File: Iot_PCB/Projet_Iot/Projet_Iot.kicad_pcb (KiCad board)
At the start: 2 copper layers, 27 parts, among them J11 110990030, J14 110990030, J17 110990030, J18 110990030, J23 110990030, J24 110990030, J36 110990030, J38 110990030, J40 110990030, J42 110990030, J8 110990030, J9 110990030, U11 FDC6326L, U6 uPesy_ESP32_Wroom_Low_Power_D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, U7 EMC2301-x-ACZL, U7 mx8v1_74LS151

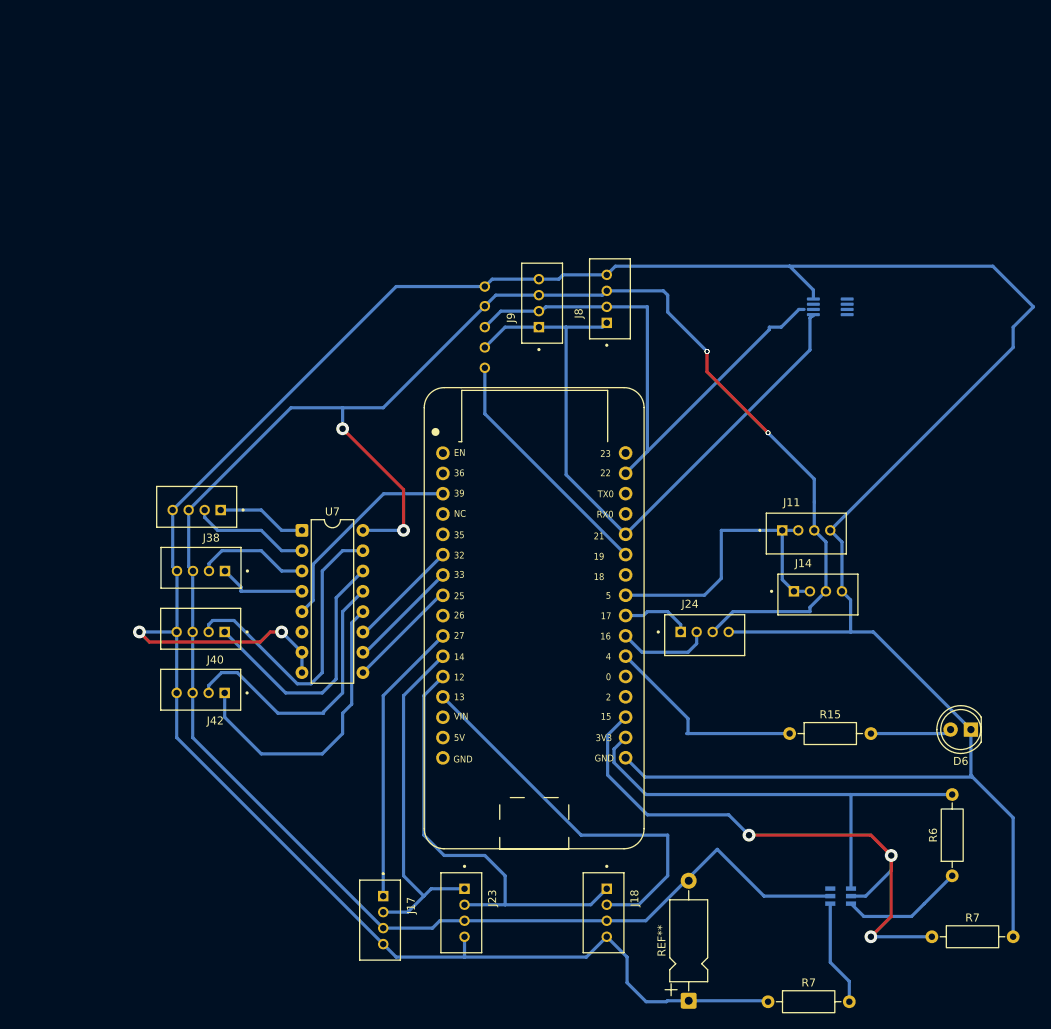
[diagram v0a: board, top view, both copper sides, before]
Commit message: final version of pcb
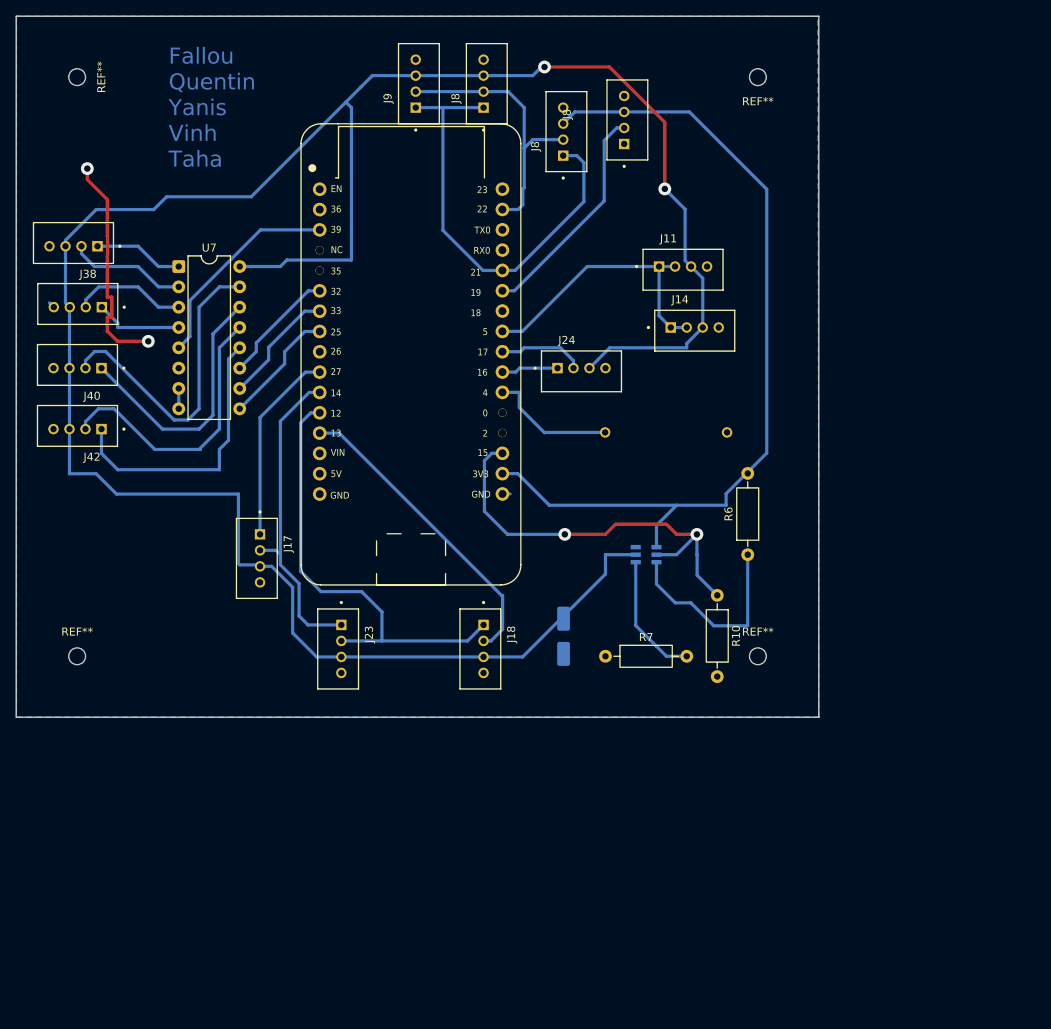
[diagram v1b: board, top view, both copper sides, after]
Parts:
- removed the ? at (71.3, 52.8)
- removed the ? at (71.3, 60.5)
- removed the ? at (71.3, 50.3)
- removed the ? at (71.3, 57.9)
- removed the ? at (71.3, 55.4)
- removed D6: LED, LED_THT:LED_D5.0mm
- removed R15: 10000, Resistor_THT:R_Axial_DIN0207_L6.3mm_D2.5mm_P10.16mm_Horizontal
- removed the R7 at (127.2, 131.6)
- removed the R7 at (106.7, 139.7)
- removed the REF** at (96.8, 139.6)
- removed the U7 at (114.5, 52.8)
- added ?: , , F.Cu at (101.6, 68.5)
- added ?: , , F.Cu at (86.3, 68.5)
- added J8: 110990030, Grove:SEEED_110990030, F.Cu at (81.1, 30.9)
- added J8: 110990030, Grove:SEEED_110990030, F.Cu at (88.7, 29.5)
- added R10: 4700, Resistor_THT:R_Axial_DIN0207_L6.3mm_D2.5mm_P10.16mm_Horizontal, F.Cu at (100.3, 88.9)
- added R7: 100, Resistor_THT:R_Axial_DIN0207_L6.3mm_D2.5mm_P10.16mm_Horizontal, F.Cu at (86.4, 96.5)
- added REF**: MountingHole_2.1mm, MountingHole:MountingHole_2.1mm, F.Cu at (20.3, 24.1)
- added REF**: MountingHole_2.1mm, MountingHole:MountingHole_2.1mm, F.Cu at (105.4, 24.1)
- added REF**: MountingHole_2.1mm, MountingHole:MountingHole_2.1mm, F.Cu at (20.3, 96.5)
- added REF**: MountingHole_2.1mm, MountingHole:MountingHole_2.1mm, F.Cu at (105.4, 96.5)
- added REF**: CP_Elec_5x3, Capacitor_SMD:CP_Elec_5x3, B.Cu at (81.1, 94.0)
- moved U11 49.1 mm to (91.4, 83.8)
- moved J17 47.8 mm to (43.2, 84.3)
- moved R6 47.6 mm to (104.1, 83.8)
- moved J14 36.4 mm to (97.5, 55.4)
- moved J18 36.4 mm to (71.1, 95.6)
- moved J23 36.4 mm to (53.3, 95.6)
- moved J24 36.4 mm to (83.4, 60.5)
- moved J36 36.4 mm to (20.4, 52.9)
- moved J40 36.4 mm to (20.4, 60.5)
- moved J42 36.4 mm to (20.4, 68.1)
- moved U6 36.4 mm to (62.0, 57.1)
- moved U7 36.4 mm to (33.0, 47.8)
- moved J11 36.4 mm to (96.1, 47.8)
- moved J38 36.4 mm to (19.9, 45.3)
- moved J9 31.5 mm to (62.6, 24.9)
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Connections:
- J24 pad 1: Net-(U6-GPIO17) -> Net-(U6-GPIO16)
- J24 pad 2: Net-(U6-GPIO16) -> Net-(U6-GPIO17)
- U6 pad 2: /ADC1 -> unconnected-(U6-GPIO39-Pad3)
- U6 pad 3: unconnected-(U6-GPIO39-Pad3) -> /ADC2
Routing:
- net /GND: track 440.3 -> 32.6 mm
- net /3v3_ESP: track 59.4 -> 107.6 mm
- net /SDL: track 70.4 -> 34.8 mm
- net /intterupt_ia: track 30.6 -> 0.00 mm
- net /interrupt_ia: track 0.00 -> 28.1 mm
- net /SDA: track 82.6 -> 54.9 mm
- net /Enable_LS: track 74.9 -> 52.5 mm, vias 3 -> 2
- net /Grove1-1: track 35.6 -> 24.4 mm
- net /Grove3-3: track 49.5 -> 38.5 mm
- net Net-(D6-A): track 10.2 -> 0.00 mm
- net Net-(U11-R1,C1): track 15.4 -> 25.2 mm
- net Net-(U6-GPIO4): track 25.8 -> 16.1 mm
- net /3v3: track 281.6 -> 290.1 mm, vias 7 -> 2
- net Net-(U6-GPIO16): track 11.6 -> 7.08 mm
- net /Grove1-2: track 44.4 -> 40.2 mm
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- added copper zone on B.Cu, net /GND
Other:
- board outline added: 100.3 x 87.6 mm
- board text added: "BUZZER IHM"
- board text added: "Capteur de température"
- board text added: "Fallou Quentin Yanis Vinh Taha"
- board text removed: "Capteur de température sol"

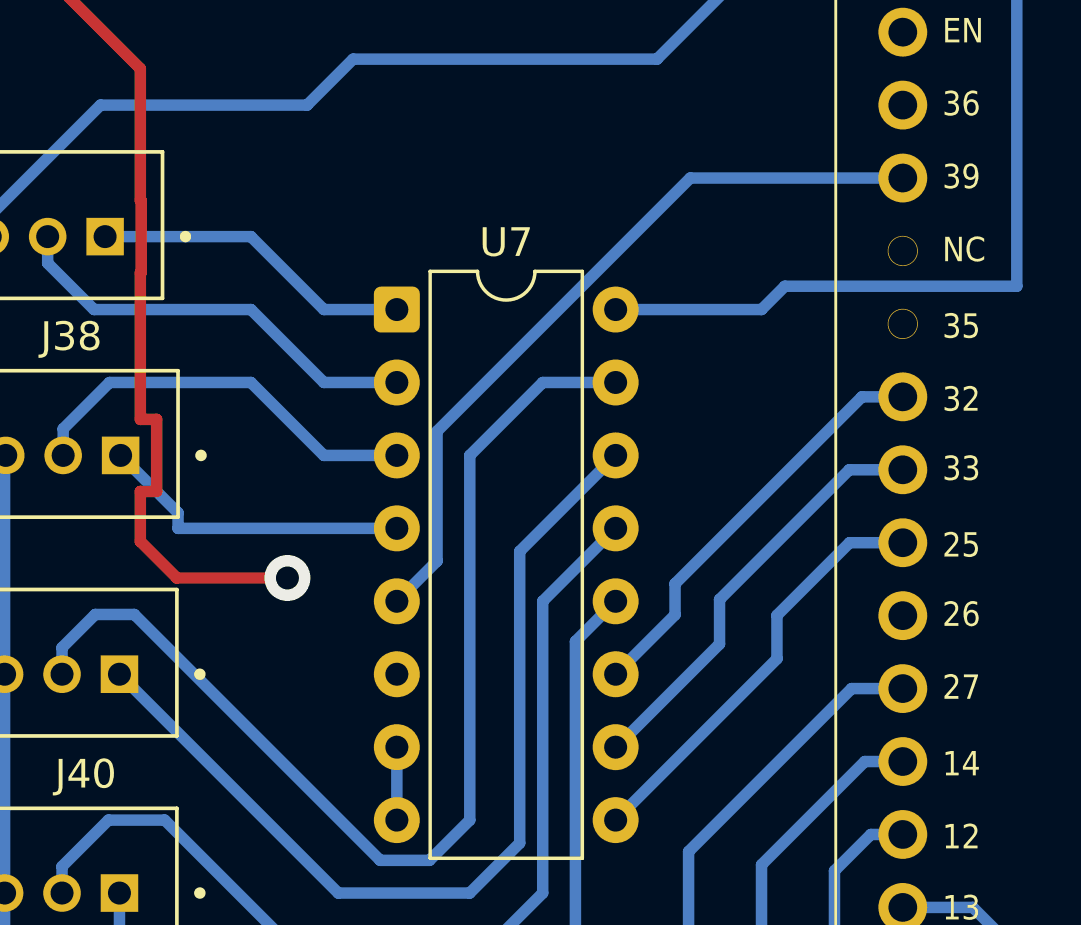
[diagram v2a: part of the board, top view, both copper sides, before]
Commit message: correction pcb final
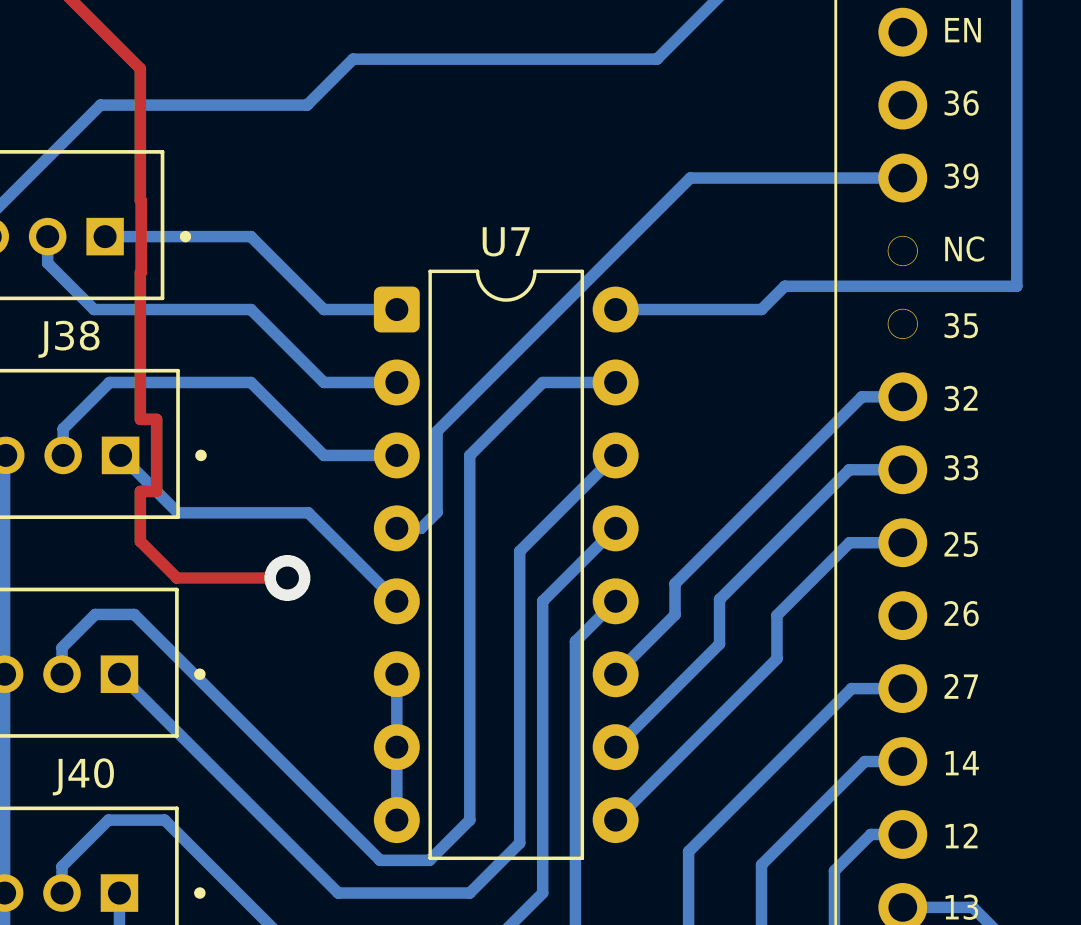
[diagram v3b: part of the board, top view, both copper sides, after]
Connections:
- U7 pad 4: /Mux8v1_capt_hum1/Hum0 -> /ADC2
- U7 pad 5: /ADC2 -> /Mux8v1_capt_hum1/Hum0
- U7 pad 6: unconnected-(U7-~{Z}-Pad6) -> /GND
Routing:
- net /GND: track 32.6 -> 35.1 mm
- net /ADC2: track 26.4 -> 24.3 mm
- net /Mux8v1_capt_hum1/Hum0: track 11.0 -> 11.7 mm
